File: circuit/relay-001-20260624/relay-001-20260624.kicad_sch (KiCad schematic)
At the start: 14 parts, among them J1 Conn_01x03_Pin, J10 Conn_01x02_Pin, J11 Conn_01x02_Pin, J12 Conn_01x02_Pin, J13 Conn_01x02_Pin, J14 Conn_01x02_Pin, J2 Conn_02x05_Odd_Even, J3 Conn_02x08_Odd_Even, J4 Conn_02x09_Odd_Even, J5 Conn_01x02_Pin, J6 Conn_01x02_Pin, J7 Conn_01x02_Pin, J8 Conn_01x02_Pin, J9 Conn_01x02_Pin

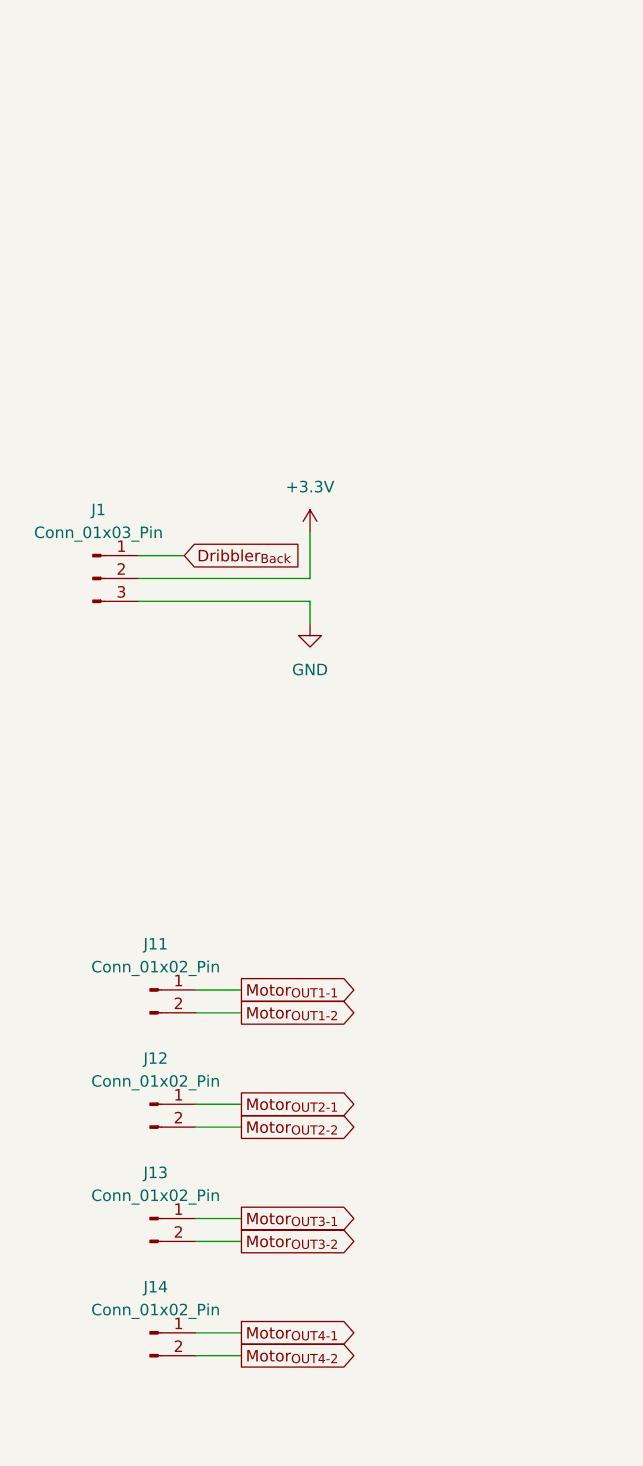
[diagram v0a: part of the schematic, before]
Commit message: Update 供給基板のボード図を進めた
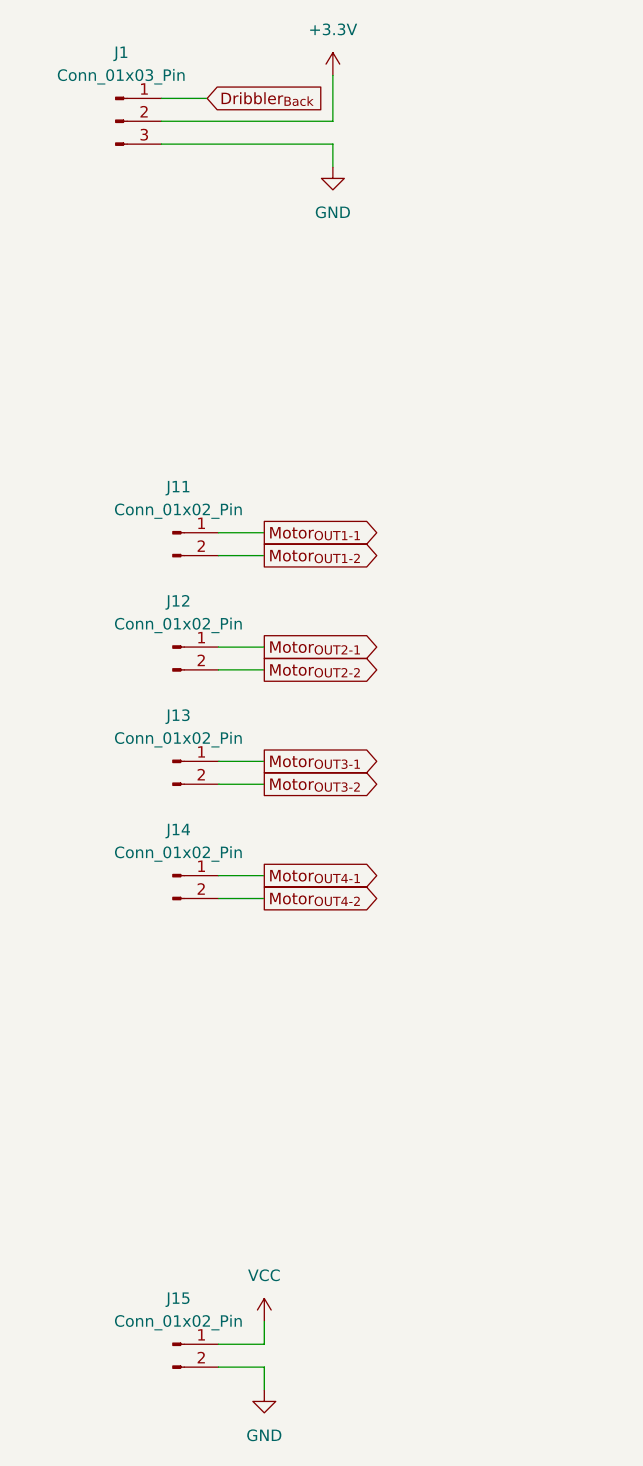
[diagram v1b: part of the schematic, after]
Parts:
- added J15: Conn_01x02_Pin, Connector_JST:JST_XH_B2B-XH-A_1x02_P2.50mm_Vertical, symbol Connector:Conn_01x02_Pin
- J1: footprint (none) -> Connector_PinHeader_2.54mm:PinHeader_1x03_P2.54mm_Vertical
- J10: footprint (none) -> Connector_AMASS:AMASS_XT30PW-M_1x02_P2.50mm_Horizontal
- J11, J12, J13, J14, J9: footprint (none) -> Connector_JST:JST_XH_B2B-XH-A_1x02_P2.50mm_Vertical
- J2: footprint (none) -> Connector_PinSocket_2.54mm:PinSocket_2x05_P2.54mm_Vertical
- J3: footprint (none) -> Connector_PinSocket_2.54mm:PinSocket_2x08_P2.54mm_Horizontal
- J4: footprint (none) -> Connector_PinSocket_2.54mm:PinSocket_2x09_P2.54mm_Vertical
- J5, J6, J7, J8: footprint (none) -> Connector_AMASS:AMASS_XT30U-M_1x02_P5.0mm_Vertical
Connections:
- net GND: now also J15.2 (Pin_2)
- net VCC: now also J15.1 (Pin_1)
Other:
- moved on the sheet: J1, J11, J12, J13, J14

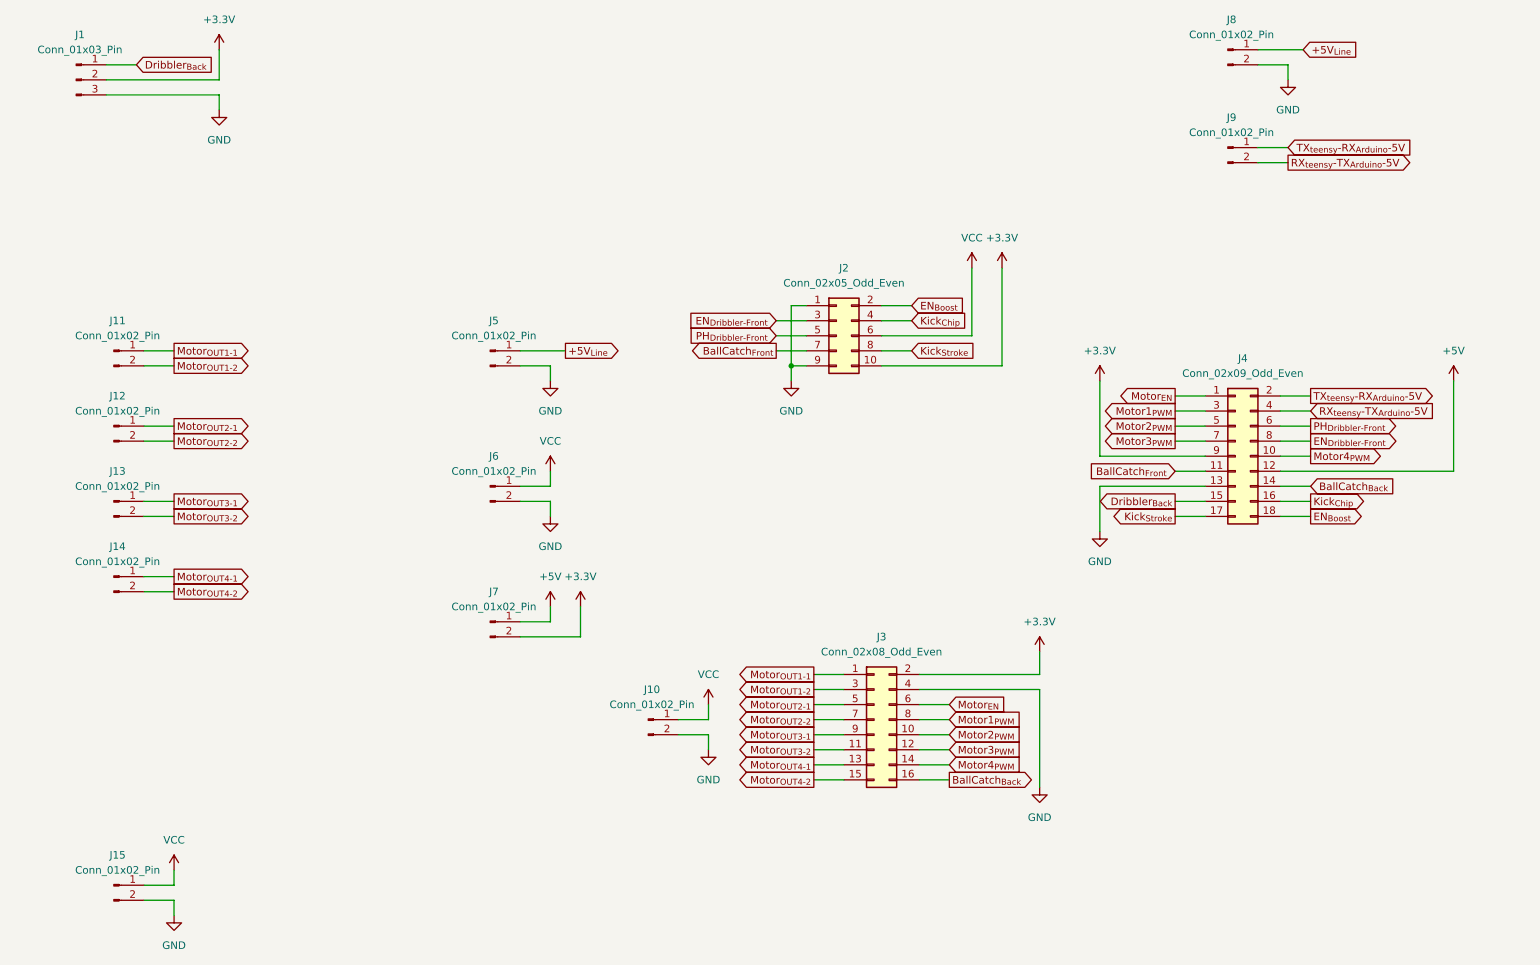
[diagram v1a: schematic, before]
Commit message: Update 供給基板のボード図を進めた
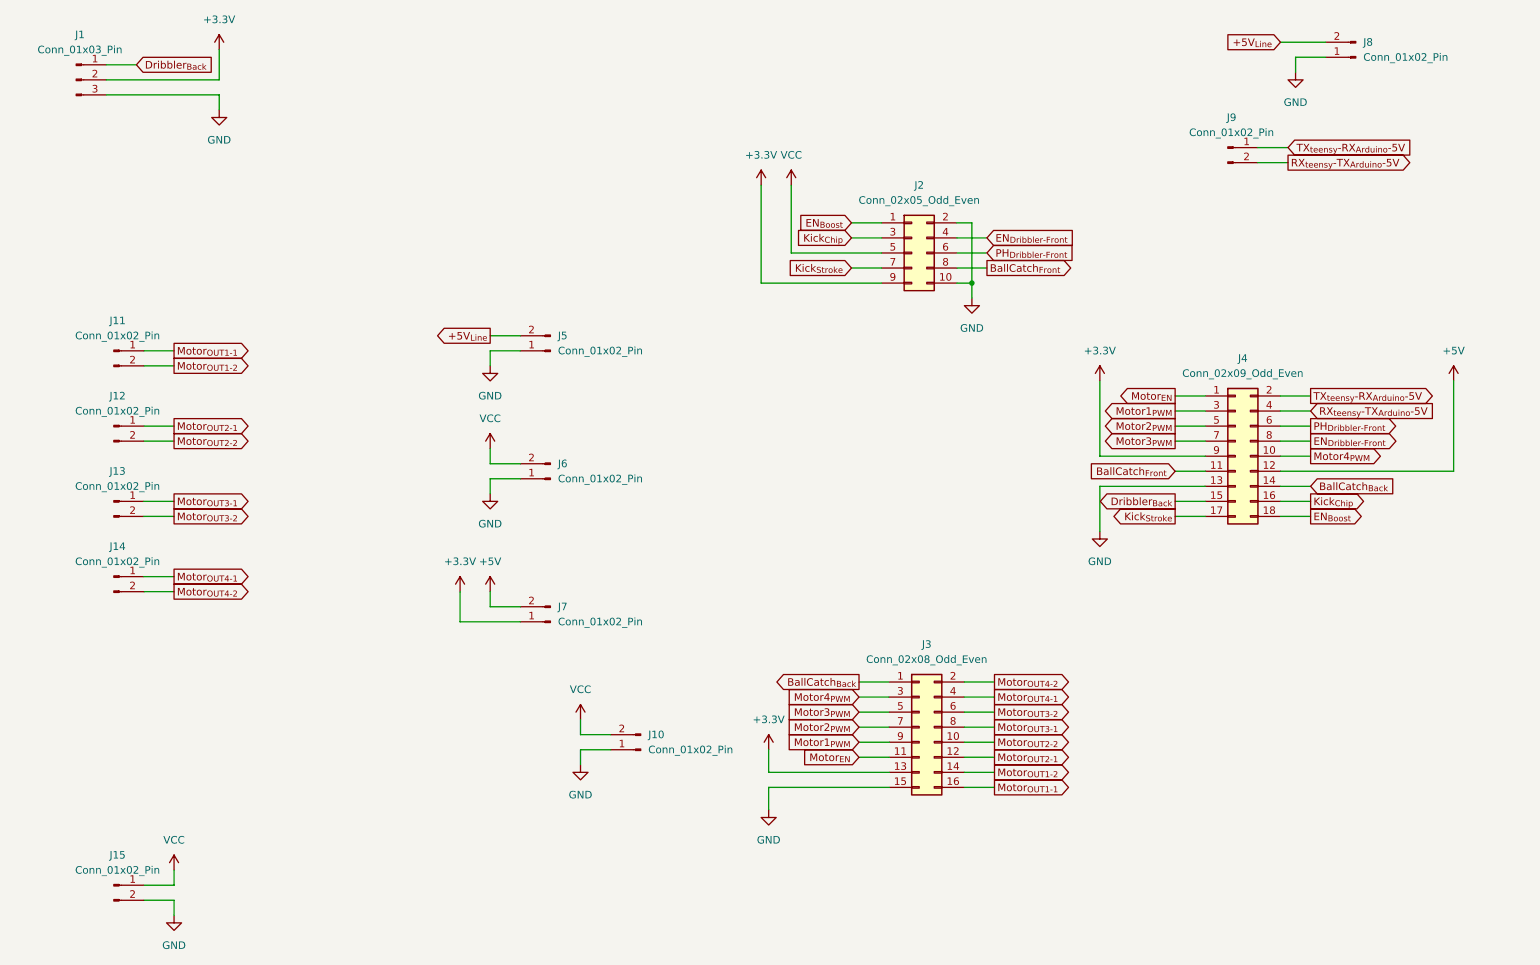
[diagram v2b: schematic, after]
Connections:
- net +3.3V: now also J2.9 (Pin_9), J3.13 (Pin_13), J7.1 (Pin_1); no longer J2.10 (Pin_10), J3.2 (Pin_2), J7.2 (Pin_2)
- net +5V: now also J7.2 (Pin_2); no longer J7.1 (Pin_1)
- net +5V_{Line}: now also J5.2 (Pin_2), J8.2 (Pin_2); no longer J5.1 (Pin_1), J8.1 (Pin_1)
- net BallCatch_{Back}: now also J3.1 (Pin_1); no longer J3.16 (Pin_16)
- net BallCatch_{Front}: now also J2.8 (Pin_8); no longer J2.7 (Pin_7)
- net EN_{Boost}: now also J2.1 (Pin_1); no longer J2.2 (Pin_2)
- net EN_{Dribbler-Front}: now also J2.4 (Pin_4); no longer J2.3 (Pin_3)
- net GND: now also J10.1 (Pin_1), J2.10 (Pin_10), J2.2 (Pin_2), J3.15 (Pin_15), J5.1 (Pin_1), J6.1 (Pin_1), J8.1 (Pin_1); no longer J10.2 (Pin_2), J2.1 (Pin_1), J2.9 (Pin_9), J3.4 (Pin_4), J5.2 (Pin_2), J6.2 (Pin_2), J8.2 (Pin_2)
- net Kick_{Chip}: now also J2.3 (Pin_3); no longer J2.4 (Pin_4)
- net Kick_{Stroke}: now also J2.7 (Pin_7); no longer J2.8 (Pin_8)
- net Motor1_{PWM}: now also J3.9 (Pin_9); no longer J3.8 (Pin_8)
- net Motor2_{PWM}: now also J3.7 (Pin_7); no longer J3.10 (Pin_10)
- net Motor3_{PWM}: now also J3.5 (Pin_5); no longer J3.12 (Pin_12)
- net Motor4_{PWM}: now also J3.3 (Pin_3); no longer J3.14 (Pin_14)
- net Motor_{EN}: now also J3.11 (Pin_11); no longer J3.6 (Pin_6)
- net Motor_{OUT1-1}: now also J3.16 (Pin_16); no longer J3.1 (Pin_1)
- net Motor_{OUT1-2}: now also J3.14 (Pin_14); no longer J3.3 (Pin_3)
- net Motor_{OUT2-1}: now also J3.12 (Pin_12); no longer J3.5 (Pin_5)
- net Motor_{OUT2-2}: now also J3.10 (Pin_10); no longer J3.7 (Pin_7)
- net Motor_{OUT3-1}: now also J3.8 (Pin_8); no longer J3.9 (Pin_9)
- net Motor_{OUT3-2}: now also J3.6 (Pin_6); no longer J3.11 (Pin_11)
- net Motor_{OUT4-1}: now also J3.4 (Pin_4); no longer J3.13 (Pin_13)
- net Motor_{OUT4-2}: now also J3.2 (Pin_2); no longer J3.15 (Pin_15)
- net PH_{Dribbler-Front}: now also J2.6 (Pin_6); no longer J2.5 (Pin_5)
- net VCC: now also J10.2 (Pin_2), J2.5 (Pin_5), J6.2 (Pin_2); no longer J10.1 (Pin_1), J2.6 (Pin_6), J6.1 (Pin_1)
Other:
- moved on the sheet: J10, J2, J3, J5, J6, J7, J8
